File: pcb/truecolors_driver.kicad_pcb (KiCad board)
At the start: 4 copper layers, 70 x 90 mm, 88 parts, among them CN1 1.0-3PWT, CN2 47053-1000, Q1 AOD413A(UMW), Q2 AOD413A(UMW), Q3 AOD413A(UMW), Q4 BSS138, SW1 TS-1088-AR02016, U1 AP63205WU-7, U2 CH224A, U3 ESP32-S3-WROOM-1(N8R8), U4 AMS1117-3.3, U5 LM3409MY/NOPB, U6 LM3409MY/NOPB, U7 LM3409MY/NOPB

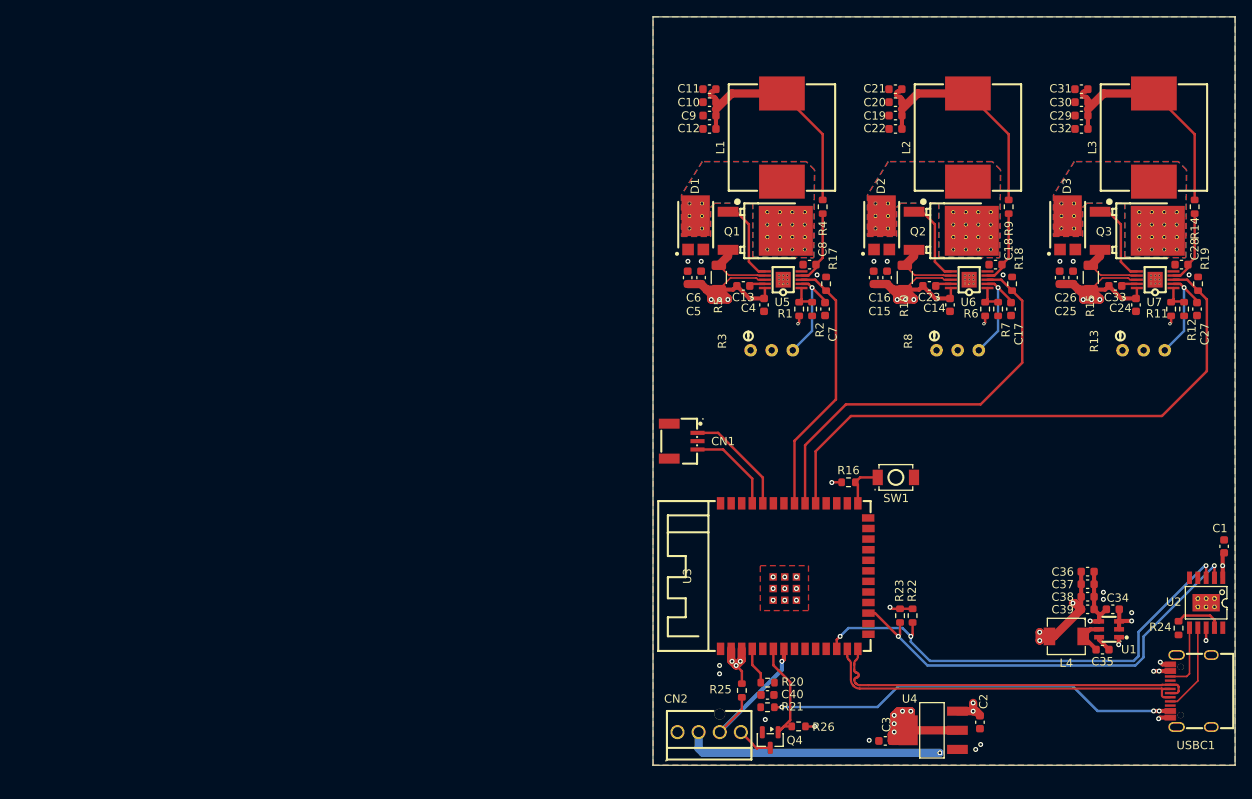
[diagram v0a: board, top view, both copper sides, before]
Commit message: add mic, add ntc, fix all drc errors
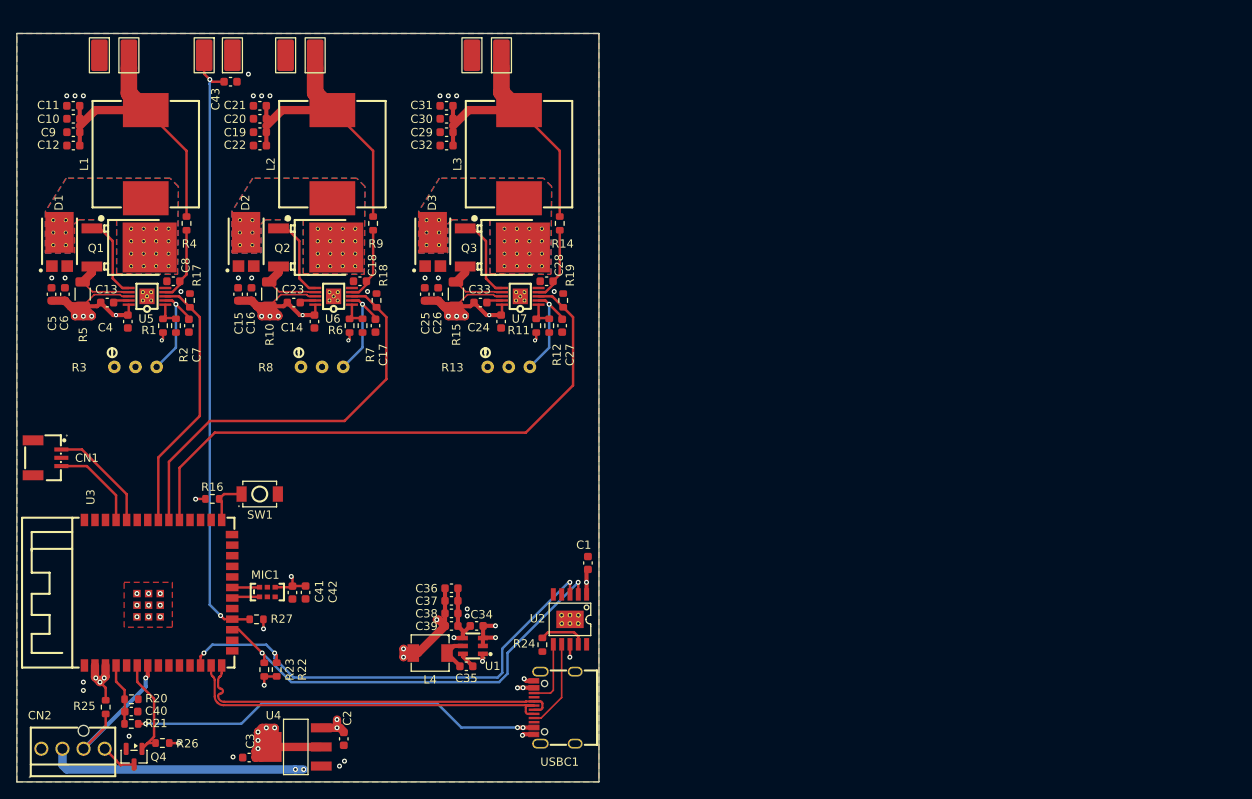
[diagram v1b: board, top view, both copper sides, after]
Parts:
- added C41: 100nF 16V, Capacitor_SMD:C_0603_1608Metric, F.Cu at (93.6, 122.2)
- added C42: 10uF 25V, Capacitor_SMD:C_0603_1608Metric, F.Cu at (95.2, 122.2)
- added C43: 100nF 16V, Capacitor_SMD:C_0603_1608Metric, F.Cu at (86.2, 60.8)
- added MIC1: MSM261DGT003, EasyEDA:MIC-SMD_6P-L4.0-W2.0_LMD4020T261-OC3, F.Cu at (90.6, 122.2)
- added R27: 10k, Resistor_SMD:R_0603_1608Metric, F.Cu at (89.3, 125.4)
- added TP1: NTC+, TestPoint:TestPoint_Keystone_5019_Miniature, F.Cu at (83.0, 57.6)
- added TP2: NTC-, TestPoint:TestPoint_Keystone_5019_Miniature, F.Cu at (86.4, 57.6)
- added TP3: R+, TestPoint:TestPoint_Keystone_5019_Miniature, F.Cu at (74.0, 57.6)
- added TP4: GND, TestPoint:TestPoint_Keystone_5019_Miniature, F.Cu at (70.4, 57.6)
- added TP5: G+, TestPoint:TestPoint_Keystone_5019_Miniature, F.Cu at (96.4, 57.6)
- added TP6: GND, TestPoint:TestPoint_Keystone_5019_Miniature, F.Cu at (92.8, 57.6)
- added TP7: B+, TestPoint:TestPoint_Keystone_5019_Miniature, F.Cu at (118.8, 57.6)
- added TP8: GND, TestPoint:TestPoint_Keystone_5019_Miniature, F.Cu at (115.2, 57.6)
- moved R22 76.7 mm to (91.7, 131.5), turned to 90 degrees
- moved R23 76.7 mm to (90.3, 131.5), turned to 90 degrees
- moved C13 76.5 mm to (71.4, 87.4)
- moved C8 76.5 mm to (79.3, 84.8)
- moved R2 76.5 mm to (79.6, 90.1)
- moved R3 76.5 mm to (74.8, 95.1)
- moved SW1 76.5 mm to (89.7, 110.4)
- moved U1 76.5 mm to (115.3, 128.7)
- moved C1 76.5 mm to (129.2, 118.7)
- moved C11 76.5 mm to (67.3, 63.7)
- moved C2 76.5 mm to (99.8, 139.8)
- moved C3 76.5 mm to (88.4, 142.1)
- moved C35 76.5 mm to (114.6, 131.1)
- moved C4 76.5 mm to (73.8, 89.6)
- moved C40 76.5 mm to (74.3, 136.5)
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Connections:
- net Net-(U3-IO0) renamed /BOOT
- U3 pad 18: unconnected-(U3-IO10-Pad18) -> /NTC_ADC
- U3 pad 20: unconnected-(U3-IO12-Pad20) -> /MIC_CLK
- U3 pad 21: unconnected-(U3-IO13-Pad21) -> /MIC_DATA
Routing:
- net /NTC_ADC: track 0.00 -> 73.7 mm, vias 0 -> 2
- net +3.3V: track 37.6 -> 43.5 mm, vias 11 -> 13
- net /driverB/VOUT: track 29.2 -> 34.3 mm
- net /driverG/VOUT: track 29.2 -> 34.3 mm
- net /driverR/VOUT: track 29.2 -> 34.3 mm
- net /MIC_CLK: track 0.00 -> 3.33 mm
- net /MIC_DATA: track 0.00 -> 3.29 mm
- net /VIN_ADC: track 4.48 -> 7.48 mm
- net +20V: track 135.7 -> 137.2 mm
- net +5V: vias 7 -> 8
- net GND: vias 29 -> 39
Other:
- rule pad_to_mask_clearance: 0 -> 0.05

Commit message: refactor schematic
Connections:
- net /CC1 renamed /power/CC1
- net /CC2 renamed /power/CC2
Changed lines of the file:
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@@
 		)
 		(property ki_fp_filters "C_*")
-		(sheetname "/")
-		(sheetfile "truecolors_driver.kicad_sch")
+		(sheetname "/power/")
+		(sheetfile "power.kicad_sch")
 		(units
 			(unit
@@
 		)
 		(property ki_fp_filters "R_*")
-		(sheetname "/")
-		(sheetfile "truecolors_driver.kicad_sch")
+		(sheetname "/power/")
+		(sheetfile "power.kicad_sch")
 		(units
 			(unit
@@
 		)
 		(property ki_fp_filters "R_*")
-		(sheetname "/")
-		(sheetfile "truecolors_driver.kicad_sch")
+		(sheetname "/power/")
+		(sheetfile "power.kicad_sch")
 		(units
 			(unit
@@
 		)
 		(property ki_fp_filters "C_*")
-		(sheetname "/")
-		(sheetfile "truecolors_driver.kicad_sch")
+		(sheetname "/power/")
+		(sheetfile "power.kicad_sch")
 		(units
 			(unit
@@
 		(sheetname "/driverB/")
 		(sheetfile "numb12_driver.kicad_sch")
+		(units
+			(unit
+				(name "A")
+				(pins "1" "2" "3" "4" "5" "11" "10" "9" "8" "7" "6")
+			)
+		)
 		(attr smd)
 		(duplicate_pad_numbers_are_jumpers no)
@@
 		)
 		(property ki_fp_filters "C_*")
-		(sheetname "/")
-		(sheetfile "truecolors_driver.kicad_sch")
+		(sheetname "/power/")
+		(sheetfile "power.kicad_sch")
 		(units
 			(unit
@@
 			)
 		)
-		(sheetname "/")
-		(sheetfile "truecolors_driver.kicad_sch")
+		(sheetname "/power/")
+		(sheetfile "power.kicad_sch")
 		(units
 			(unit
@@
 		(sheetname "/driverR/")
 		(sheetfile "numb12_driver.kicad_sch")
+		(units
+			(unit
+				(name "A")
+				(pins "1" "2" "3" "4" "5" "11" "10" "9" "8" "7" "6")
+			)
+		)
 		(attr smd)
 		(duplicate_pad_numbers_are_jumpers no)
@@
 		)
 		(property ki_fp_filters "C_*")
-		(sheetname "/")
-		(sheetfile "truecolors_driver.kicad_sch")
+		(sheetname "/power/")
+		(sheetfile "power.kicad_sch")
 		(units
 			(unit
@@
 		(sheetname "/")
 		(sheetfile "truecolors_driver.kicad_sch")
+		(units
+			(unit
+				(name "A")
+				(pins "1" "2" "3" "4")
+			)
+		)
 		(attr through_hole)
 		(duplicate_pad_numbers_are_jumpers no)
@@
 		)
 		(property ki_fp_filters "C_*")
-		(sheetname "/")
-		(sheetfile "truecolors_driver.kicad_sch")
+		(sheetname "/power/")
+		(sheetfile "power.kicad_sch")
 		(units
 			(unit
@@
 		(sheetname "/driverG/")
 		(sheetfile "numb12_driver.kicad_sch")
+		(units
+			(unit
+				(name "A")
+				(pins "1" "2" "3" "4" "5" "11" "10" "9" "8" "7" "6")
+			)
+		)
 		(attr smd)
 		(duplicate_pad_numbers_are_jumpers no)
@@
 		)
 		(property ki_fp_filters "C_*")
-		(sheetname "/")
-		(sheetfile "truecolors_driver.kicad_sch")
+		(sheetname "/power/")
+		(sheetfile "power.kicad_sch")
 		(units
 			(unit
@@
 			)
 		)
-		(sheetname "/")
-		(sheetfile "truecolors_driver.kicad_sch")
+		(sheetname "/power/")
+		(sheetfile "power.kicad_sch")
+		(units
+			(unit
+				(name "A")
+				(pins "1" "2" "3" "4" "5" "11" "10" "9" "8" "7" "6")
+			)
+		)
 		(attr smd)
 		(duplicate_pad_numbers_are_jumpers no)
@@
 			(size 1.5 0.6)
 			(layers "F.Cu" "F.Mask" "F.Paste")
-			(net "/CC2")
+			(net "/power/CC2")
 			(pinfunction "CC2_6")
 			(pintype "unspecified")
@@
 			(size 1.5 0.6)
 			(layers "F.Cu" "F.Mask" "F.Paste")
-			(net "/CC1")
+			(net "/power/CC1")
 			(pinfunction "CC1_7")
 			(pintype "unspecified")
@@
 			)
 		)
-		(sheetname "/")
-		(sheetfile "truecolors_driver.kicad_sch")
+		(sheetname "/power/")
+		(sheetfile "power.kicad_sch")
 		(units
 			(unit
@@
 		)
 		(property ki_fp_filters "R_*")
-		(sheetname "/")
-		(sheetfile "truecolors_driver.kicad_sch")
+		(sheetname "/power/")
+		(sheetfile "power.kicad_sch")
 		(units
 			(unit
@@
 			)
 		)
-		(sheetname "/")
-		(sheetfile "truecolors_driver.kicad_sch")
+		(sheetname "/power/")
+		(sheetfile "power.kicad_sch")
 		(units
 			(unit
@@
 		)
 		(property ki_fp_filters "C_*")
-		(sheetname "/")
-		(sheetfile "truecolors_driver.kicad_sch")
+		(sheetname "/power/")
+		(sheetfile "power.kicad_sch")
 		(units
 			(unit
@@
 			(net "unconnected-(U3-IO5-Pad5)")
 			(pinfunction "IO5_5")
-			(pintype "unspecified")
+			(pintype "unspecified+no_connect")
 		)
 		(pad "6" smd rect
@@
 			(net "unconnected-(U3-IO15-Pad8)")
 			(pinfunction "IO15_8")
-			(pintype "unspecified")
+			(pintype "unspecified+no_connect")
 		)
 		(pad "9" smd rect
@@
 			(net "unconnected-(U3-IO16-Pad9)")
 			(pinfunction "IO16_9")
-			(pintype "unspecified")
+			(pintype "unspecified+no_connect")
 		)
 		(pad "10" smd rect
@@
 			(net "unconnected-(U3-IO17-Pad10)")
 			(pinfunction "IO17_10")
-			(pintype "unspecified")
+			(pintype "unspecified+no_connect")
 		)
 		(pad "11" smd rect
@@
 			(net "unconnected-(U3-IO18-Pad11)")
 			(pinfunction "IO18_11")
-			(pintype "unspecified")
+			(pintype "unspecified+no_connect")
 		)
 		(pad "12" smd rect
@@
 			(net "unconnected-(U3-IO3-Pad15)")
 			(pinfunction "IO3_15")
-			(pintype "unspecified")
+			(pintype "unspecified+no_connect")
 		)
 		(pad "16" smd rect
@@
 			(net "unconnected-(U3-IO46-Pad16)")
 			(pinfunction "IO46_16")
-			(pintype "unspecified")
+			(pintype "unspecified+no_connect")
 		)
 		(pad "17" smd rect
@@
 			(net "unconnected-(U3-IO11-Pad19)")
 			(pinfunction "IO11_19")
-			(pintype "unspecified")
+			(pintype "unspecified+no_connect")
 		)
 		(pad "20" smd rect
@@
 			(net "unconnected-(U3-IO14-Pad22)")
 			(pinfunction "IO14_22")
-			(pintype "unspecified")
+			(pintype "unspecified+no_connect")
 		)
 		(pad "23" smd rect
@@
 			(net "unconnected-(U3-IO21-Pad23)")
 			(pinfunction "IO21_23")
-			(pintype "unspecified")
+			(pintype "unspecified+no_connect")
 		)
 		(pad "24" smd rect
@@
 			(net "unconnected-(U3-IO47-Pad24)")
 			(pinfunction "IO47_24")
-			(pintype "unspecified")
+			(pintype "unspecified+no_connect")
 		)
 		(pad "25" smd rect
@@
 			(net "unconnected-(U3-IO48-Pad25)")
 			(pinfunction "IO48_25")
-			(pintype "unspecified")
+			(pintype "unspecified+no_connect")
 		)
 		(pad "26" smd rect
@@
 			(net "unconnected-(U3-IO45-Pad26)")
 			(pinfunction "IO45_26")
-			(pintype "unspecified")
+			(pintype "unspecified+no_connect")
 		)
 		(pad "27" smd rect
@@
 			(net "unconnected-(U3-IO35-Pad28)")
 			(pinfunction "IO35_28")
-			(pintype "unspecified")
+			(pintype "unspecified+no_connect")
 		)
 		(pad "29" smd rect
@@
 			(net "unconnected-(U3-IO36-Pad29)")
 			(pinfunction "IO36_29")
-			(pintype "unspecified")
+			(pintype "unspecified+no_connect")
 		)
 		(pad "30" smd rect
@@
 			(net "unconnected-(U3-IO37-Pad30)")
 			(pinfunction "IO37_30")
-			(pintype "unspecified")
+			(pintype "unspecified+no_connect")
 		)
 		(pad "31" smd rect
@@
 			(net "unconnected-(U3-IO41-Pad34)")
 			(pinfunction "IO41_34")
-			(pintype "unspecified")
+			(pintype "unspecified+no_connect")
 		)
 		(pad "35" smd rect
@@
 			(net "unconnected-(U3-IO42-Pad35)")
 			(pinfunction "IO42_35")
-			(pintype "unspecified")
+			(pintype "unspecified+no_connect")
 		)
 		(pad "36" smd rect
@@
 			(net "unconnected-(U3-IO2-Pad38)")
 			(pinfunction "IO2_38")
-			(pintype "unspecified")
+			(pintype "unspecified+no_connect")
 		)
 		(pad "39" smd rect
@@
 			(net "unconnected-(U3-IO1-Pad39)")
 			(pinfunction "IO1_39")
-			(pintype "unspecified")
+			(pintype "unspecified+no_connect")
 		)
 		(pad "40" smd rect
@@
 			)
 		)
-		(sheetname "/")
-		(sheetfile "truecolors_driver.kicad_sch")
+		(sheetname "/power/")
+		(sheetfile "power.kicad_sch")
+		(units
+			(unit
+				(name "A")
+				(pins "A1B12" "A4B9" "B8" "A5" "B7" "A6" "A7" "B6" "A8" "B5" "B4A9" "B1A12"
+					"4" "3" "2" "1"
+				)
+			)
+		)
 		(attr smd)
 		(duplicate_pad_numbers_are_jumpers no)
@@
 			(size 0.3 1.3)
 			(layers "F.Cu" "F.Mask" "F.Paste")
-			(net "/CC1")
+			(net "/power/CC1")
 			(pinfunction "CC1_A5")
 			(pintype "unspecified")
@@
 			(size 0.3 1.3)
 			(layers "F.Cu" "F.Mask" "F.Paste")
-			(net "/CC2")
+			(net "/power/CC2")
 			(pinfunction "CC2_B5")
 			(pintype "unspecified")
@@
 		)
 		(property ki_fp_filters "C_*")
-		(sheetname "/")
-		(sheetfile "truecolors_driver.kicad_sch")
+		(sheetname "/power/")
+		(sheetfile "power.kicad_sch")
 		(units
 			(unit
@@
 		)
 		(property ki_fp_filters "C_*")
-		(sheetname "/")
-		(sheetfile "truecolors_driver.kicad_sch")
+		(sheetname "/power/")
+		(sheetfile "power.kicad_sch")
 		(units
 			(unit
@@
 	)
 	(segment
-		(start 124.68 134.32)
-		(end 125.015348 133.984652)
-		(width 0.2)
-		(layer "F.Cu")
-		(net "/CC2")
-	)
-	(segment
-		(start 122.7 134.32)
-		(end 124.68 134.32)
-		(width 0.2)
-		(layer "F.Cu")
-		(net "/CC2")
-	)
-	(segment
-		(start 125.015348 133.984652)
-		(end 125.015348 128.454788)
-		(width 0.2)
-		(layer "F.Cu")
-		(net "/CC2")
-	)
-	(segment
-		(start 126.015348 128.454788)
-		(end 126.015348 134.854652)
-		(width 0.2)
-		(layer "F.Cu")
-		(net "/CC1")
-	)
-	(segment
-		(start 123.55 137.32)
-		(end 122.7 137.32)
-		(width 0.2)
-		(layer "F.Cu")
-		(net "/CC1")
-	)
-	(segment
-		(start 126.015348 134.854652)
-		(end 123.55 137.32)
-		(width 0.2)
-		(layer "F.Cu")
-		(net "/CC1")
-	)
-	(segment
 		(start 122.7 135.82)
 		(end 121.724999 135.82)
@@
 		(net "/BOOT")
 	)
+	(segment
+		(start 124.68 134.32)
+		(end 125.015348 133.984652)
+		(width 0.2)
+		(layer "F.Cu")
+		(net "/power/CC2")
+	)
+	(segment
+		(start 122.7 134.32)
+		(end 124.68 134.32)
+		(width 0.2)
+		(layer "F.Cu")
+		(net "/power/CC2")
+	)
+	(segment
+		(start 125.015348 133.984652)
+		(end 125.015348 128.454788)
+		(width 0.2)
+		(layer "F.Cu")
+		(net "/power/CC2")
+	)
+	(segment
+		(start 126.015348 128.454788)
+		(end 126.015348 134.854652)
+		(width 0.2)
+		(layer "F.Cu")
+		(net "/power/CC1")
+	)
+	(segment
+		(start 123.55 137.32)
+		(end 122.7 137.32)
+		(width 0.2)
+		(layer "F.Cu")
+		(net "/power/CC1")
+	)
+	(segment
+		(start 126.015348 134.854652)
+		(end 123.55 137.32)
+		(width 0.2)
+		(layer "F.Cu")
+		(net "/power/CC1")
+	)
 	(zone
